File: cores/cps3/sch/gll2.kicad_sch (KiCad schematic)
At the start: 1 part

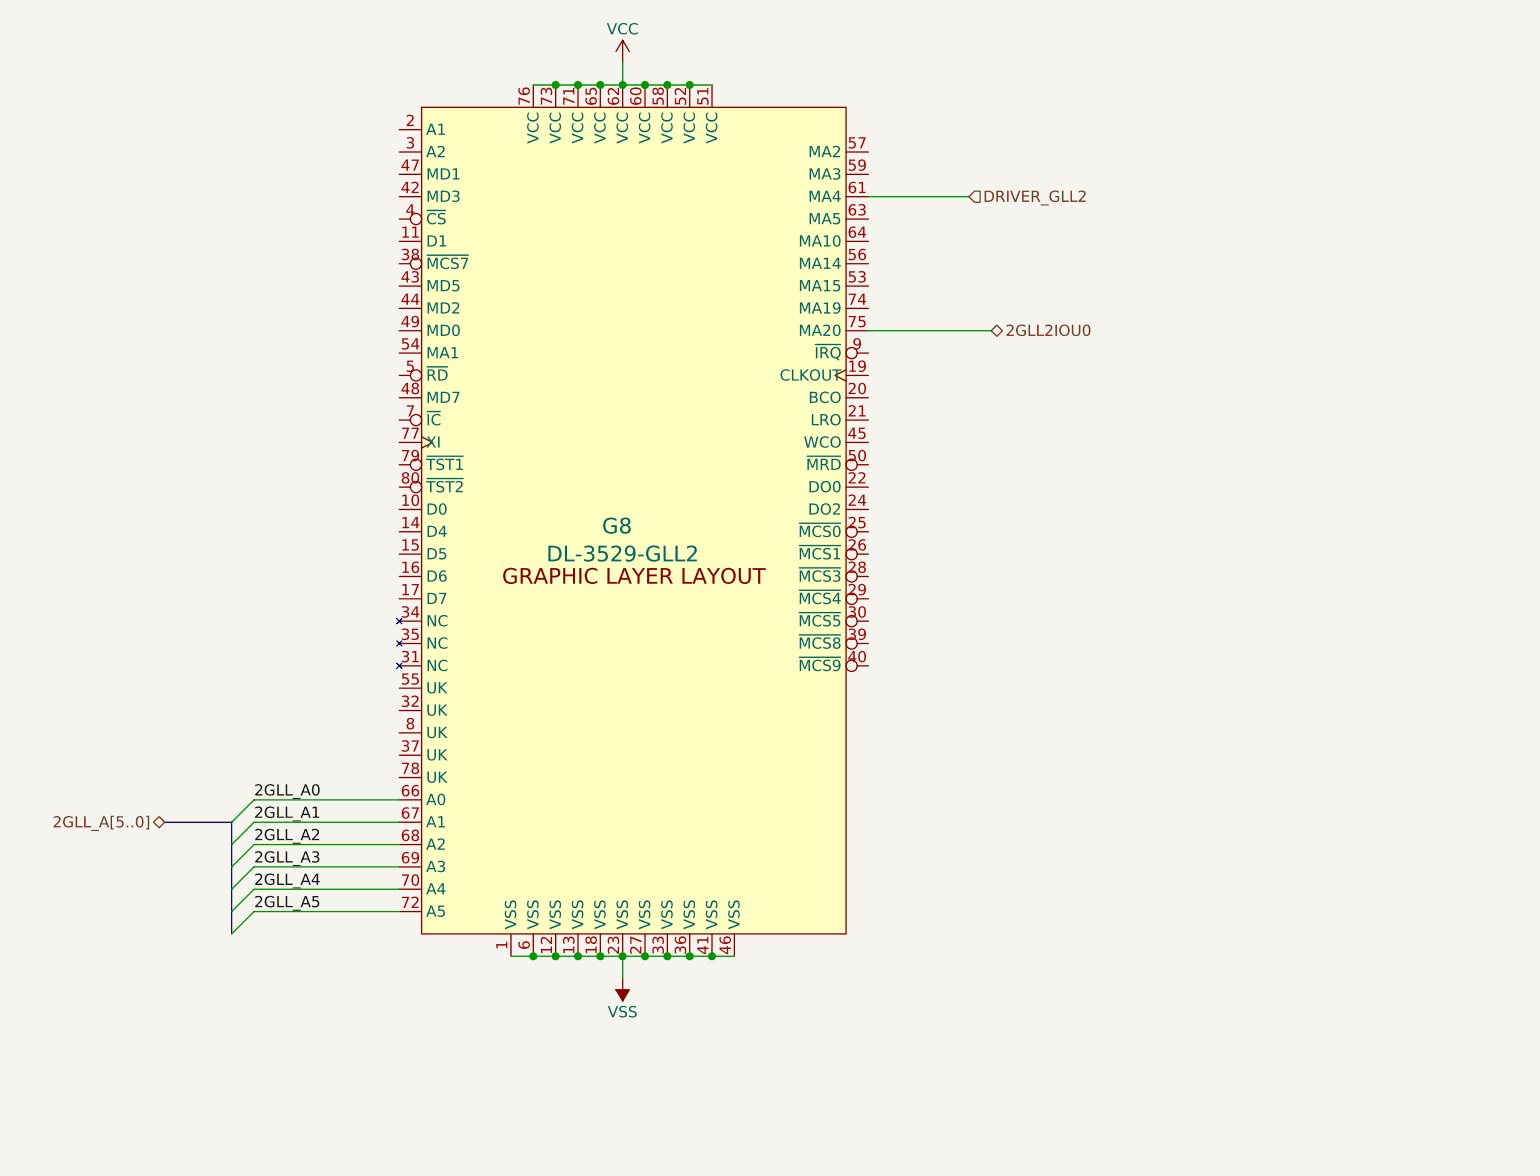
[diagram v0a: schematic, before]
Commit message: wip_ccu_gll2_cassette
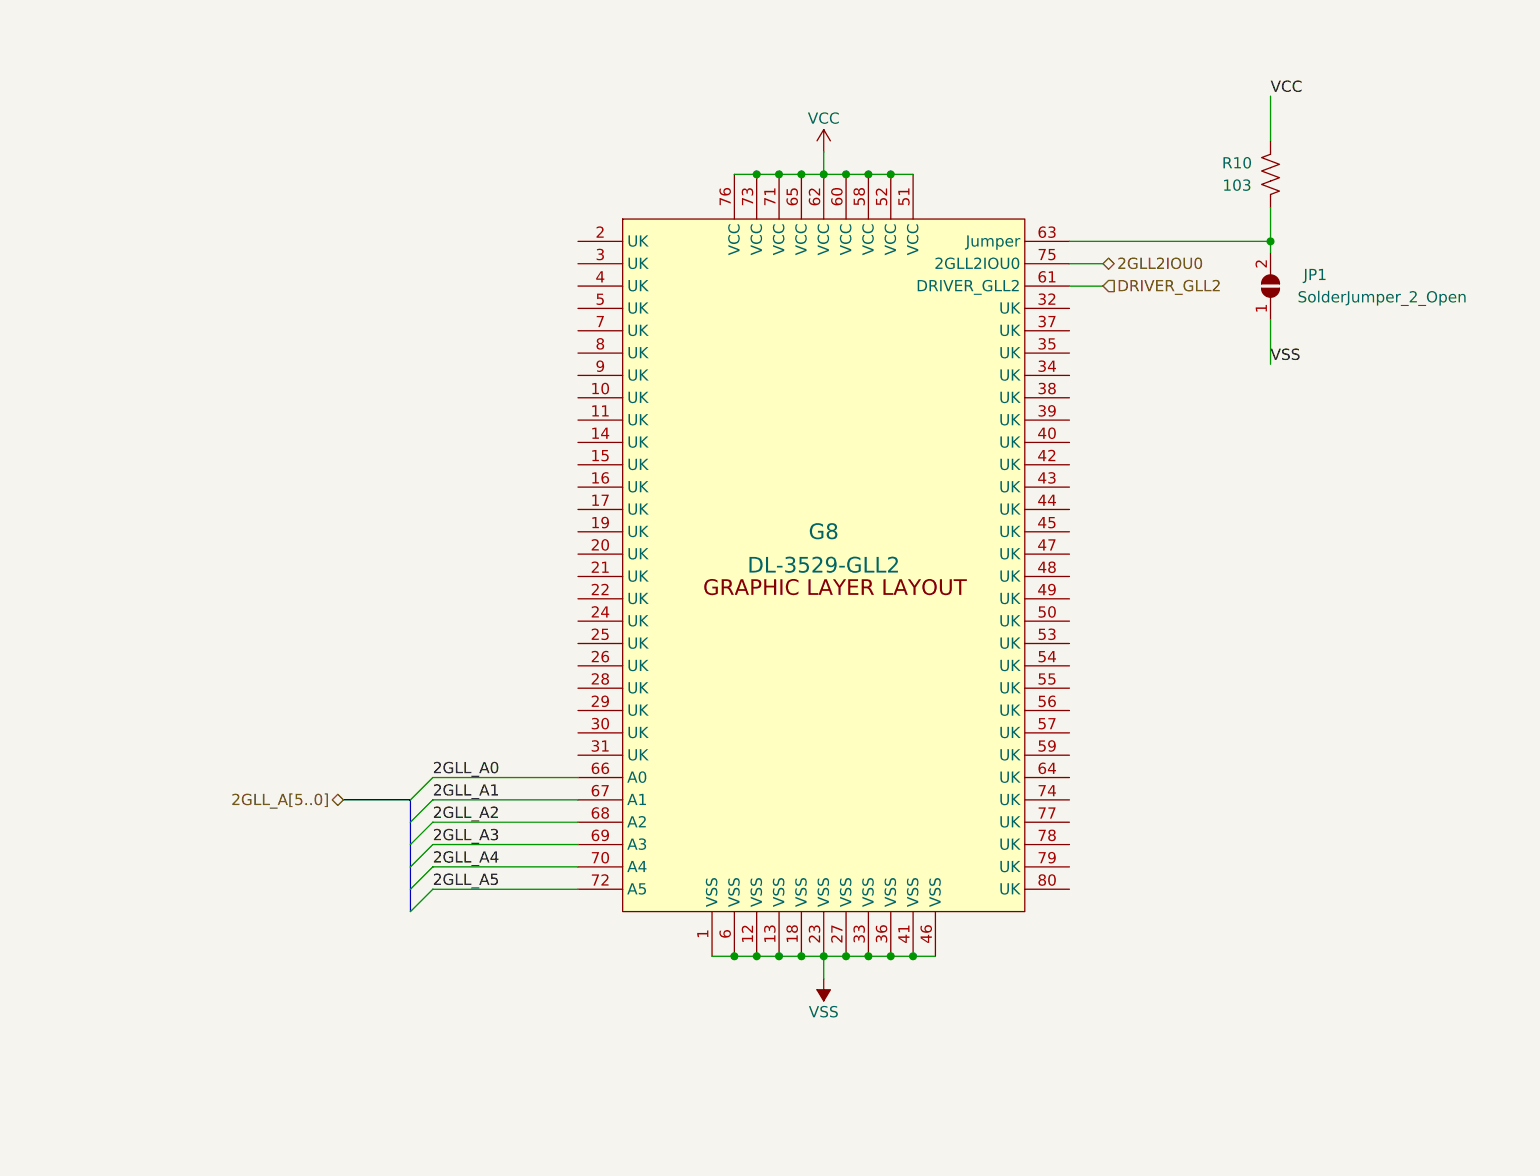
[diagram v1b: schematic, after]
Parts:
- added JP1: SolderJumper_2_Open, symbol Jumper:SolderJumper_2_Open
- added R10: 103, symbol Device:R_US
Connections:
- net VCC: now also R10.1
- net VSS: now also JP1.1 (A)
- net at G8.63 (Jumper): now also JP1.2 (B), R10.2

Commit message: wip_ccu_cassette
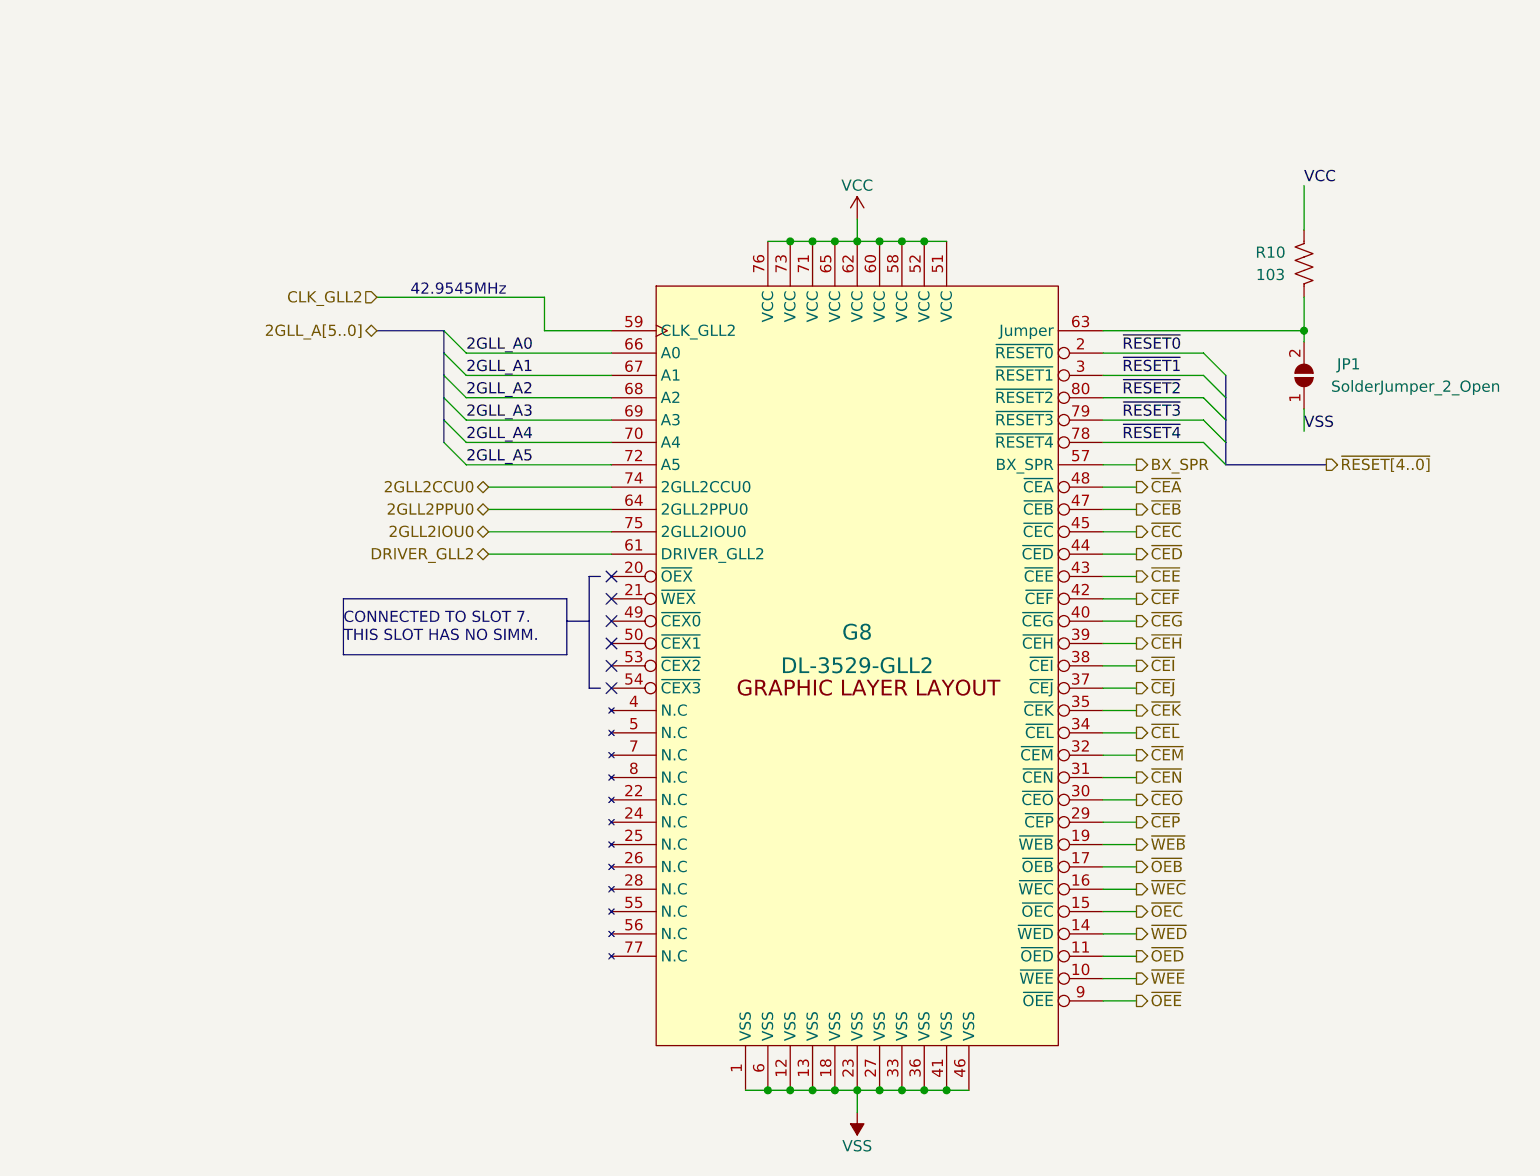
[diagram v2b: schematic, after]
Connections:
- net ~{WEE}: now reaches G8.10 (~{WEE})
- net ~{OED}: now reaches G8.11 (~{OED})
- net ~{WED}: now reaches G8.14 (~{WED})
- net ~{OEC}: now reaches G8.15 (~{OEC})
- net ~{WEC}: now reaches G8.16 (~{WEC})
- net ~{OEB}: now reaches G8.17 (~{OEB})
- net ~{WEB}: now reaches G8.19 (~{WEB})
- net ~{RESET0}: now reaches G8.2 (~{RESET0})
- net ~{CEP}: now reaches G8.29 (~{CEP})
- net ~{RESET1}: now reaches G8.3 (~{RESET1})
- net ~{CEO}: now reaches G8.30 (~{CEO})
- net ~{CEN}: now reaches G8.31 (~{CEN})
- net ~{CEM}: now reaches G8.32 (~{CEM})
- net ~{CEL}: now reaches G8.34 (~{CEL})
- net ~{CEK}: now reaches G8.35 (~{CEK})
- net ~{CEJ}: now reaches G8.37 (~{CEJ})
- net ~{CEI}: now reaches G8.38 (~{CEI})
- net ~{CEH}: now reaches G8.39 (~{CEH})
- net ~{CEG}: now reaches G8.40 (~{CEG})
- net ~{CEF}: now reaches G8.42 (~{CEF})
- net ~{CEE}: now reaches G8.43 (~{CEE})
- net ~{CED}: now reaches G8.44 (~{CED})
- net ~{CEC}: now reaches G8.45 (~{CEC})
- net ~{CEB}: now reaches G8.47 (~{CEB})
- net ~{CEA}: now reaches G8.48 (~{CEA})
- net BX_SPR: now reaches G8.57 (BX_SPR)
- net CLK_GLL2: now reaches G8.59 (CLK_GLL2)
- net 2GLL2PPU0: now reaches G8.64 (2GLL2PPU0)
- net 2GLL2CCU0: now reaches G8.74 (2GLL2CCU0)
- net ~{RESET4}: now reaches G8.78 (~{RESET4})
- net ~{RESET3}: now reaches G8.79 (~{RESET3})
- net ~{RESET2}: now reaches G8.80 (~{RESET2})
- net ~{OEE}: now reaches G8.9 (~{OEE})
- no-connect marks 0 -> 6
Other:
- note added: "42.9545MHz"
- note added: "CONNECTED TO SLOT 7. THIS SLOT HAS NO SIMM."
- moved on the sheet: JP1, R10
